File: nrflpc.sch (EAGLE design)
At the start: 68 parts, among them IC1 LPC1111/12/13/14-HVQFN33, IC2 LT1763CS8-3.3, IC3 LM3401, IC5 LM3401, IC6 LM3401, IC7 LM3401, Q1 20MHz, Q2 MOSFET-PCHANNEL, Q3 MOSFET-PCHANNEL, Q4 MOSFET-PCHANNEL, Q5 MOSFET-PCHANNEL

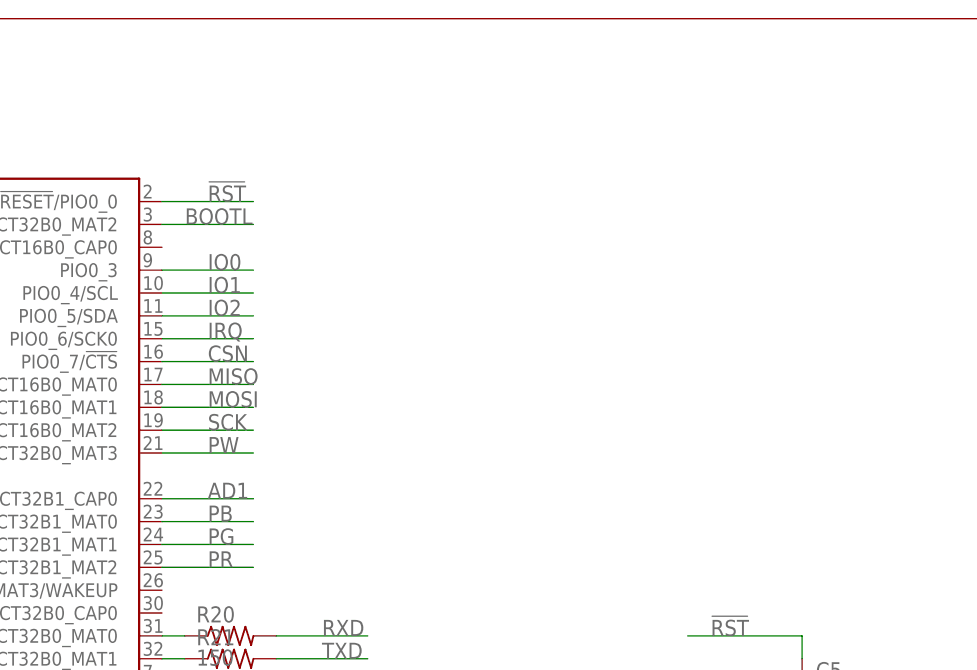
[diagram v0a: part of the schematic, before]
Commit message: Almost final routing
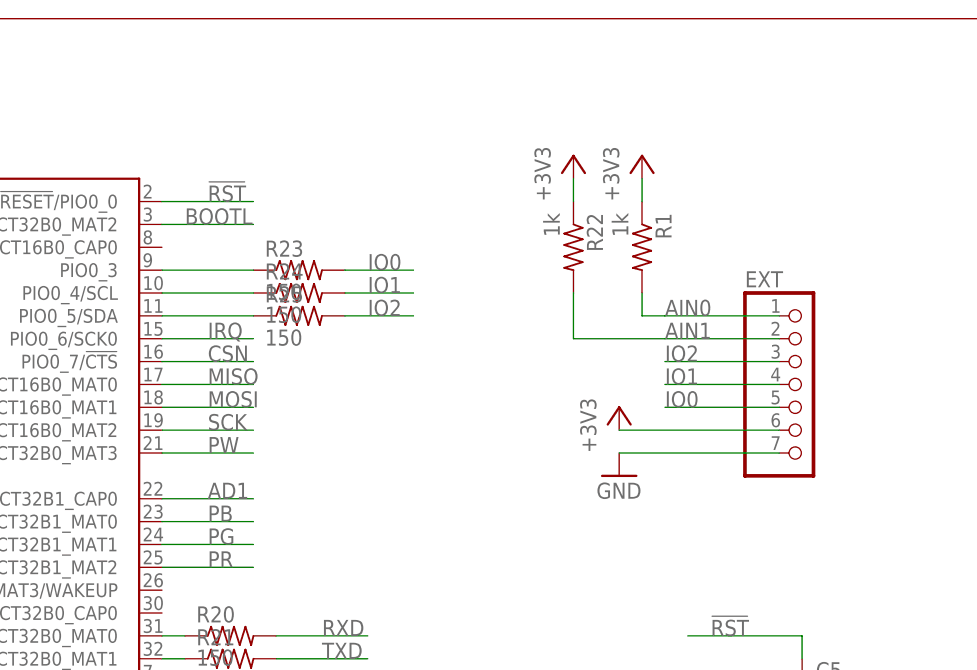
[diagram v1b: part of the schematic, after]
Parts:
- added EXT: (no value), pinhead:PINHD-1X7
- added R1, R22: 1k, rcl:R-US_R0402
- added R23, R24, R25: 150, rcl:R-US_R0402
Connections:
- new net N$34: IC1.PIO0_3, R23.1
- new net N$35: IC1.PIO0_4/SCL, R24.1
- new net N$36: IC1.PIO0_5/SDA, R25.1
- net +3V3: now also EXT.6, R1.1, R22.1
- net AIN0: now also EXT.1, R1.2
- net AIN1: now also EXT.2, R22.2
- net GND: now also EXT.7
- net IO0: now also EXT.5, R23.2; no longer IC1.PIO0_3
- net IO1: now also EXT.4, R24.2; no longer IC1.PIO0_4/SCL
- net IO2: now also EXT.3, R25.2; no longer IC1.PIO0_5/SDA
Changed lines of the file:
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@@
 <part name="C18" library="SparkFun" deviceset="CAP" device="0402-CAP" value="10nF"/>
 <part name="C17" library="rcl" deviceset="CPOL-EU" device="SMCA" value="10µF"/>
+<part name="EXT" library="pinhead" deviceset="PINHD-1X7" device=""/>
+<part name="GND16" library="supply1" deviceset="GND" device=""/>
+<part name="+3V3" library="supply1" deviceset="+3V3" device=""/>
+<part name="R1" library="rcl" deviceset="R-US_" device="R0402" value="1k"/>
+<part name="R22" library="rcl" deviceset="R-US_" device="R0402" value="1k"/>
+<part name="+3V5" library="supply1" deviceset="+3V3" device=""/>
+<part name="+3V6" library="supply1" deviceset="+3V3" device=""/>
+<part name="R23" library="rcl" deviceset="R-US_" device="R0402" value="150"/>
+<part name="R24" library="rcl" deviceset="R-US_" device="R0402" value="150"/>
+<part name="R25" library="rcl" deviceset="R-US_" device="R0402" value="150"/>
 </parts>
 <sheets>
@@
 <instance part="C18" gate="G$1" x="228.6" y="43.18" rot="R180"/>
 <instance part="C17" gate="G$1" x="238.76" y="43.18"/>
+<instance part="EXT" gate="A" x="302.26" y="177.8"/>
+<instance part="GND16" gate="1" x="281.94" y="167.64"/>
+<instance part="+3V3" gate="G$1" x="281.94" y="175.26"/>
+<instance part="R1" gate="G$1" x="284.48" y="193.04" rot="R270"/>
+<instance part="R22" gate="G$1" x="276.86" y="193.04" rot="R270"/>
+<instance part="+3V5" gate="G$1" x="276.86" y="203.2"/>
+<instance part="+3V6" gate="G$1" x="284.48" y="203.2"/>
+<instance part="R23" gate="G$1" x="246.38" y="190.5"/>
+<instance part="R24" gate="G$1" x="246.38" y="187.96"/>
+<instance part="R25" gate="G$1" x="246.38" y="185.42"/>
 </instances>
 <busses>
@@
 <wire x1="73.66" y1="139.7" x2="73.66" y2="137.16" width="0.1524" layer="91"/>
 </segment>
+<segment>
+<pinref part="EXT" gate="A" pin="7"/>
+<wire x1="281.94" y1="170.18" x2="299.72" y2="170.18" width="0.1524" layer="91"/>
+<pinref part="GND16" gate="1" pin="GND"/>
+</segment>
 </net>
 <net name="!RST" class="0">
@@
 <junction x="167.64" y="185.42"/>
 </segment>
+<segment>
+<pinref part="EXT" gate="A" pin="6"/>
+<wire x1="281.94" y1="172.72" x2="299.72" y2="172.72" width="0.1524" layer="91"/>
+<pinref part="+3V3" gate="G$1" pin="+3V3"/>
+</segment>
+<segment>
+<pinref part="R22" gate="G$1" pin="1"/>
+<pinref part="+3V5" gate="G$1" pin="+3V3"/>
+<wire x1="276.86" y1="200.66" x2="276.86" y2="198.12" width="0.1524" layer="91"/>
+</segment>
+<segment>
+<pinref part="R1" gate="G$1" pin="1"/>
+<pinref part="+3V6" gate="G$1" pin="+3V3"/>
+<wire x1="284.48" y1="198.12" x2="284.48" y2="200.66" width="0.1524" layer="91"/>
+</segment>
 </net>
 <net name="CE" class="0">
@@
 <net name="IO0" class="0">
 <segment>
-<pinref part="IC1" gate="G$1" pin="PIO0_3"/>
-<wire x1="231.14" y1="190.5" x2="241.3" y2="190.5" width="0.1524" layer="91"/>
-<label x="236.22" y="190.5" size="1.778" layer="95"/>
+<pinref part="EXT" gate="A" pin="5"/>
+<wire x1="287.02" y1="175.26" x2="299.72" y2="175.26" width="0.1524" layer="91"/>
+<label x="287.02" y="175.26" size="1.778" layer="95"/>
+</segment>
+<segment>
+<pinref part="R23" gate="G$1" pin="2"/>
+<wire x1="251.46" y1="190.5" x2="259.08" y2="190.5" width="0.1524" layer="91"/>
+<label x="254" y="190.5" size="1.778" layer="95"/>
 </segment>
 </net>
 <net name="IO1" class="0">
 <segment>
-<pinref part="IC1" gate="G$1" pin="PIO0_4/SCL"/>
-<wire x1="231.14" y1="187.96" x2="241.3" y2="187.96" width="0.1524" layer="91"/>
-<label x="236.22" y="187.96" size="1.778" layer="95"/>
+<pinref part="EXT" gate="A" pin="4"/>
+<wire x1="299.72" y1="177.8" x2="287.02" y2="177.8" width="0.1524" layer="91"/>
+<label x="287.02" y="177.8" size="1.778" layer="95"/>
+</segment>
+<segment>
+<pinref part="R24" gate="G$1" pin="2"/>
+<wire x1="251.46" y1="187.96" x2="259.08" y2="187.96" width="0.1524" layer="91"/>
+<label x="254" y="187.96" size="1.778" layer="95"/>
 </segment>
 </net>
 <net name="IO2" class="0">
 <segment>
-<pinref part="IC1" gate="G$1" pin="PIO0_5/SDA"/>
-<wire x1="231.14" y1="185.42" x2="241.3" y2="185.42" width="0.1524" layer="91"/>
-<label x="236.22" y="185.42" size="1.778" layer="95"/>
+<pinref part="EXT" gate="A" pin="3"/>
+<wire x1="299.72" y1="180.34" x2="287.02" y2="180.34" width="0.1524" layer="91"/>
+<label x="287.02" y="180.34" size="1.778" layer="95"/>
+</segment>
+<segment>
+<pinref part="R25" gate="G$1" pin="2"/>
+<wire x1="251.46" y1="185.42" x2="259.08" y2="185.42" width="0.1524" layer="91"/>
+<label x="254" y="185.42" size="1.778" layer="95"/>
 </segment>
 </net>
@@
 <label x="330.2" y="109.22" size="1.778" layer="95"/>
 </segment>
+<segment>
+<pinref part="EXT" gate="A" pin="1"/>
+<wire x1="299.72" y1="185.42" x2="287.02" y2="185.42" width="0.1524" layer="91"/>
+<label x="287.02" y="185.42" size="1.778" layer="95"/>
+<pinref part="R1" gate="G$1" pin="2"/>
+<wire x1="287.02" y1="185.42" x2="284.48" y2="185.42" width="0.1524" layer="91"/>
+<wire x1="284.48" y1="185.42" x2="284.48" y2="187.96" width="0.1524" layer="91"/>
+</segment>
 </net>
 <net name="AIN1" class="0">
@@
 <wire x1="381" y1="109.22" x2="391.16" y2="109.22" width="0.1524" layer="91"/>
 <label x="383.54" y="109.22" size="1.778" layer="95"/>
+</segment>
+<segment>
+<pinref part="EXT" gate="A" pin="2"/>
+<wire x1="299.72" y1="182.88" x2="287.02" y2="182.88" width="0.1524" layer="91"/>
+<label x="287.02" y="182.88" size="1.778" layer="95"/>
+<pinref part="R22" gate="G$1" pin="2"/>
+<wire x1="287.02" y1="182.88" x2="276.86" y2="182.88" width="0.1524" layer="91"/>
+<wire x1="276.86" y1="182.88" x2="276.86" y2="187.96" width="0.1524" layer="91"/>
 </segment>
 </net>
@@
 </segment>
 </net>
+<net name="N$34" class="0">
+<segment>
+<pinref part="IC1" gate="G$1" pin="PIO0_3"/>
+<pinref part="R23" gate="G$1" pin="1"/>
+<wire x1="231.14" y1="190.5" x2="241.3" y2="190.5" width="0.1524" layer="91"/>
+</segment>
+</net>
+<net name="N$35" class="0">
+<segment>
+<pinref part="R24" gate="G$1" pin="1"/>
+<pinref part="IC1" gate="G$1" pin="PIO0_4/SCL"/>
+<wire x1="241.3" y1="187.96" x2="231.14" y2="187.96" width="0.1524" layer="91"/>
+</segment>
+</net>
+<net name="N$36" class="0">
+<segment>
+<pinref part="IC1" gate="G$1" pin="PIO0_5/SDA"/>
+<pinref part="R25" gate="G$1" pin="1"/>
+<wire x1="231.14" y1="185.42" x2="241.3" y2="185.42" width="0.1524" layer="91"/>
+</segment>
+</net>
